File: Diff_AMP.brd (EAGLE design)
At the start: 30.2 x 16.8 mm, 22 parts, among them IC1 NCV8711ASN500T1G, IC3 MCP1501T-25E_RW, IC4 NCS21911SN2T1G, IC5 NCS21911SN2T1G

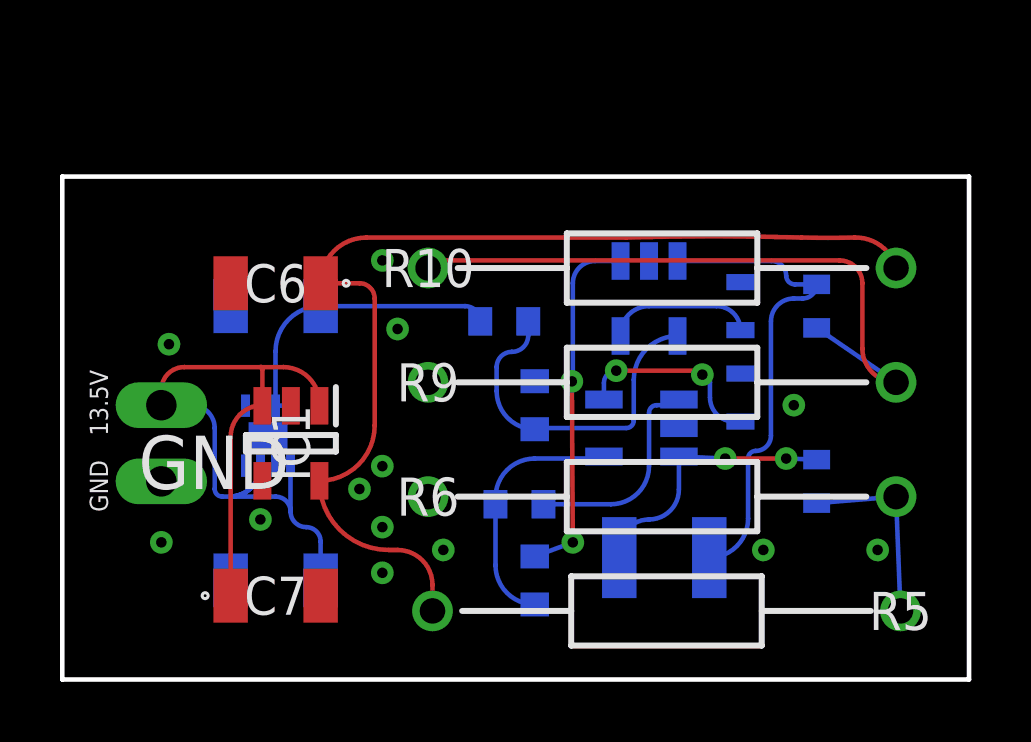
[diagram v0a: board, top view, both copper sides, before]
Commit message: rev_1
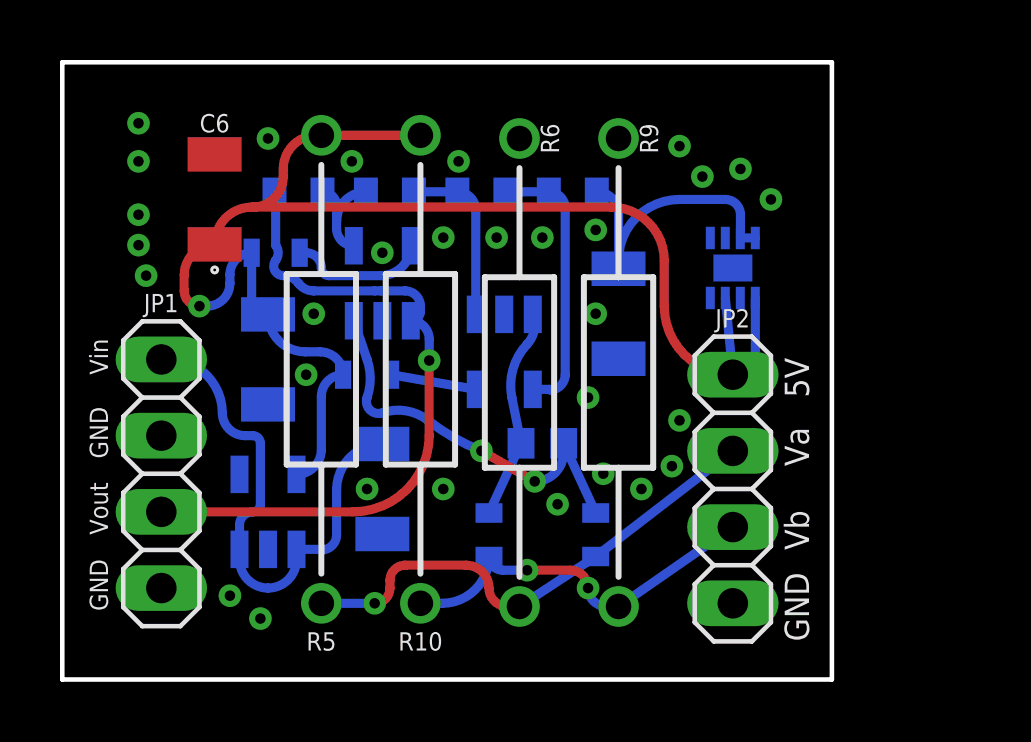
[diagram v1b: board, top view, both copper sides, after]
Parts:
- removed R7, R8: ERA-3VRW1911V, SamacSys_Parts:ERA3KV_(0603)
- added JP2: (no value), pinhead:1X04
- added R11, R12: ERA-3VEB1911V, SamacSys_Parts:ERA3KV_(0603)
- C2: value C1210C184J1JACAUTO -> GCJ188R71E183KA01J; device SamacSys_Parts:C1210 -> SamacSys_Parts:CAPC1608X100N
- JP1: device pinhead:1X02 -> pinhead:1X04
- moved R5 19.3 mm to (8.64, 2.54), turned to 90 degrees
- moved IC3 16.5 mm to (22.4, 13.7)
- moved C5 16.2 mm to (7.11, 14.2), turned to 180 degrees
- moved R4 13.8 mm to (10.9, 16.3), turned to 0 degrees
- moved R2 12.8 mm to (7.87, 16.3), turned to 0 degrees
- moved C4 12.7 mm to (10.2, 10.2), turned to 180 degrees
- moved R6 12.3 mm to (15.2, 18.0), turned to 270 degrees
- moved C1 11.4 mm to (18.5, 12.2), turned to 90 degrees
- moved R10 11.2 mm to (11.9, 2.54), turned to 90 degrees
- moved R9 10.3 mm to (18.5, 18.0), turned to 270 degrees
- moved IC5 9.89 mm to (10.7, 13.2), turned to 90 degrees
- moved C3 7.37 mm to (6.86, 10.7), turned to 90 degrees
- moved R3 7.33 mm to (14.0, 16.3), turned to 0 degrees
- moved C2 5.57 mm to (16.0, 7.87)
- moved IC4 5.14 mm to (14.7, 10.9)
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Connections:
- removed net 13.5V: C3.2, C7.1, IC1.1, IC1.3, IC3.1, IC3.3, JP1.2
- removed net N$10: C6.1, IC1.5, R10.2, R5.2
- removed net N$14: IC5.1, R2.2
- removed net N$6: R5.1, R6.2, R7.1
- removed net N$7: R10.1, R8.1, R9.2
- new net 5V: C3.2, C4.1, C5.1, C6.1, IC1.5, IC3.1, IC3.3, JP2.1, R10.2, R5.2
- new net VA: JP2.2, R12.1, R5.1, R6.2
- new net VB: JP2.3, R10.1, R11.1, R9.2
- new net VIN: C7.1, IC1.1, IC1.3, JP1.1
- new net VOUT: IC5.1, JP1.3, R2.2
- net GND: now also JP1.2, JP1.4, JP2.4; no longer C4.1, C5.1, JP1.1
- net N$3: now also C2.1, R11.2; no longer C2.2, R8.2
- net N$9: now also C2.2, R12.2; no longer C2.1, R7.2
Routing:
- net 5V: track 0.00 -> 48.1 mm, vias 0 -> 1
- net N$10: track 35.1 -> 0.00 mm
- net 13.5V: track 28.9 -> 0.00 mm
- net VOUT: track 0.00 -> 22.5 mm, vias 0 -> 1
- net N$7: track 21.9 -> 0.00 mm
- net VIN: track 0.00 -> 16.9 mm
- net VA: track 0.00 -> 16.7 mm, vias 0 -> 1
- net VB: track 0.00 -> 12.6 mm, vias 0 -> 2
- net N$3: track 15.7 -> 6.97 mm
- net N$12: track 13.1 -> 5.79 mm, vias 2 -> 0
- net N$14: track 7.00 -> 0.00 mm
- net N$6: track 6.47 -> 0.00 mm
- net N$13: track 8.28 -> 3.61 mm
- net N$9: track 8.79 -> 13.2 mm
- net GND: track 2.77 -> 0.00 mm, vias 13 -> 30
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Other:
- board size 30.2 x 16.8 mm -> 25.7 x 20.6 mm
- board text added: "5V"
- board text added: "RYAN THAI BAJA SAE 2021-2022 ELECTRICAL TEAM"
- board text added: "Va"
- board text added: "Vb"
- board text added: "Vin"
- board text added: "Vout"
- board text removed: "13.5V"
